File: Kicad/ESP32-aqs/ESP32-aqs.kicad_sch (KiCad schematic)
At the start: 28 parts, among them J2 JST connector SEN55, J3 ufl connector, J4 UART Connector, SW1 TC-1102-B-C-B, SW2 TC-1102-B-C-B, U1 LD1117S33TR_SOT223, U2 ESP32-WROOM-32, U3 SGP41-D-R4, U4 SX1276S8S+T-X1

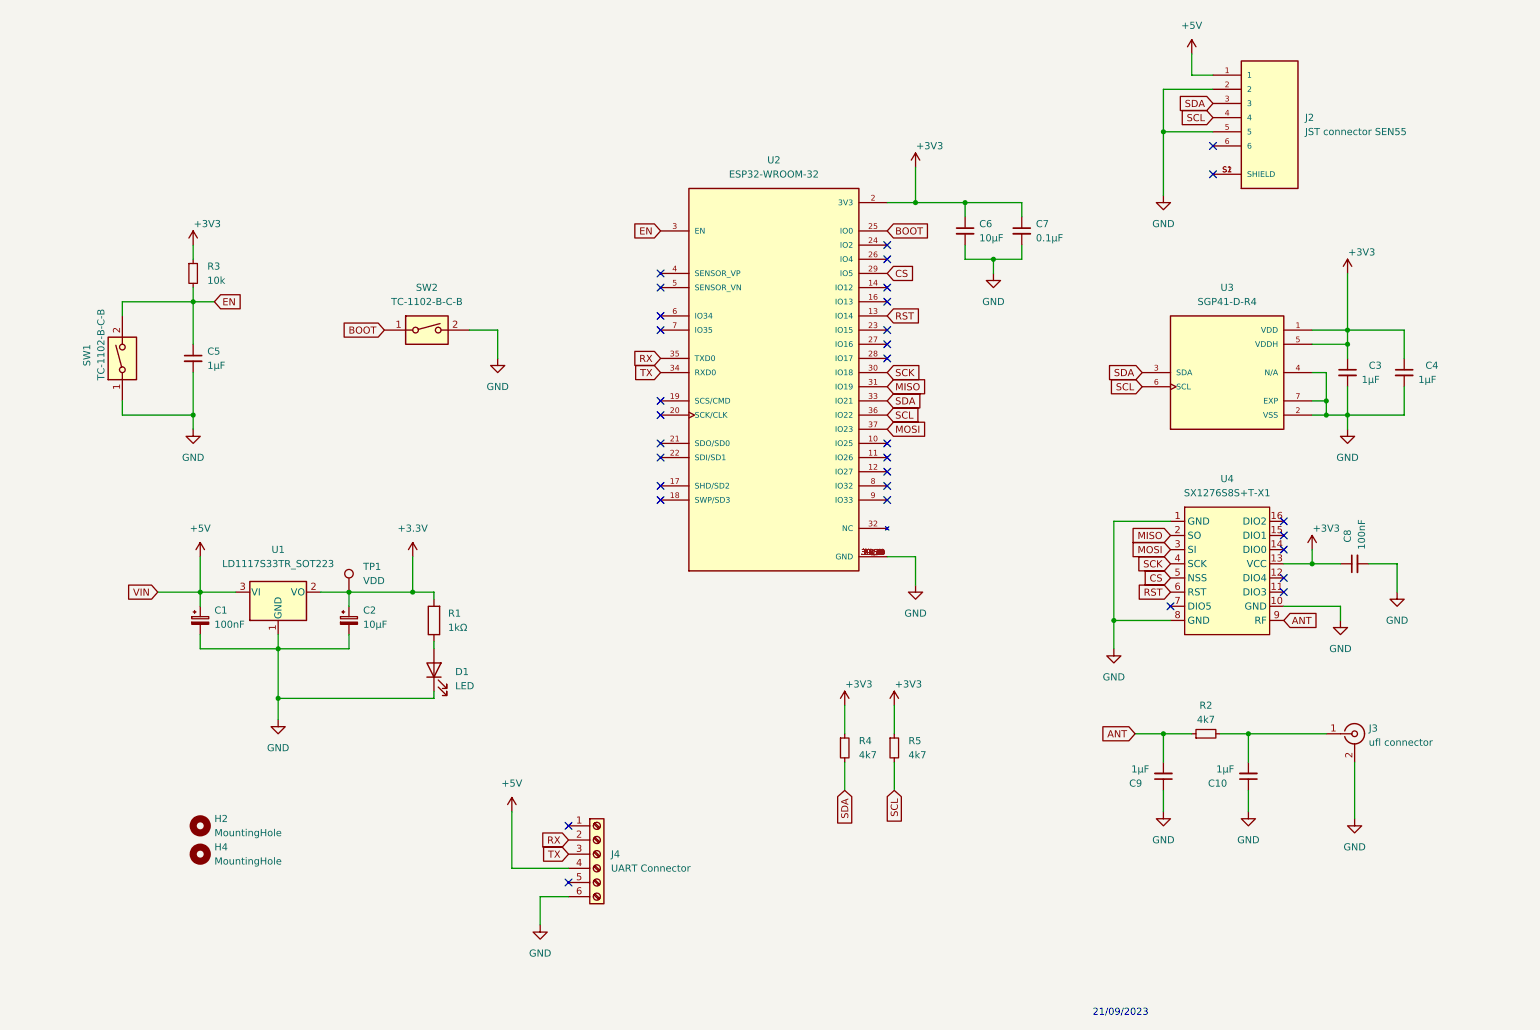
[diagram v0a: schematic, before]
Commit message: schematic v2
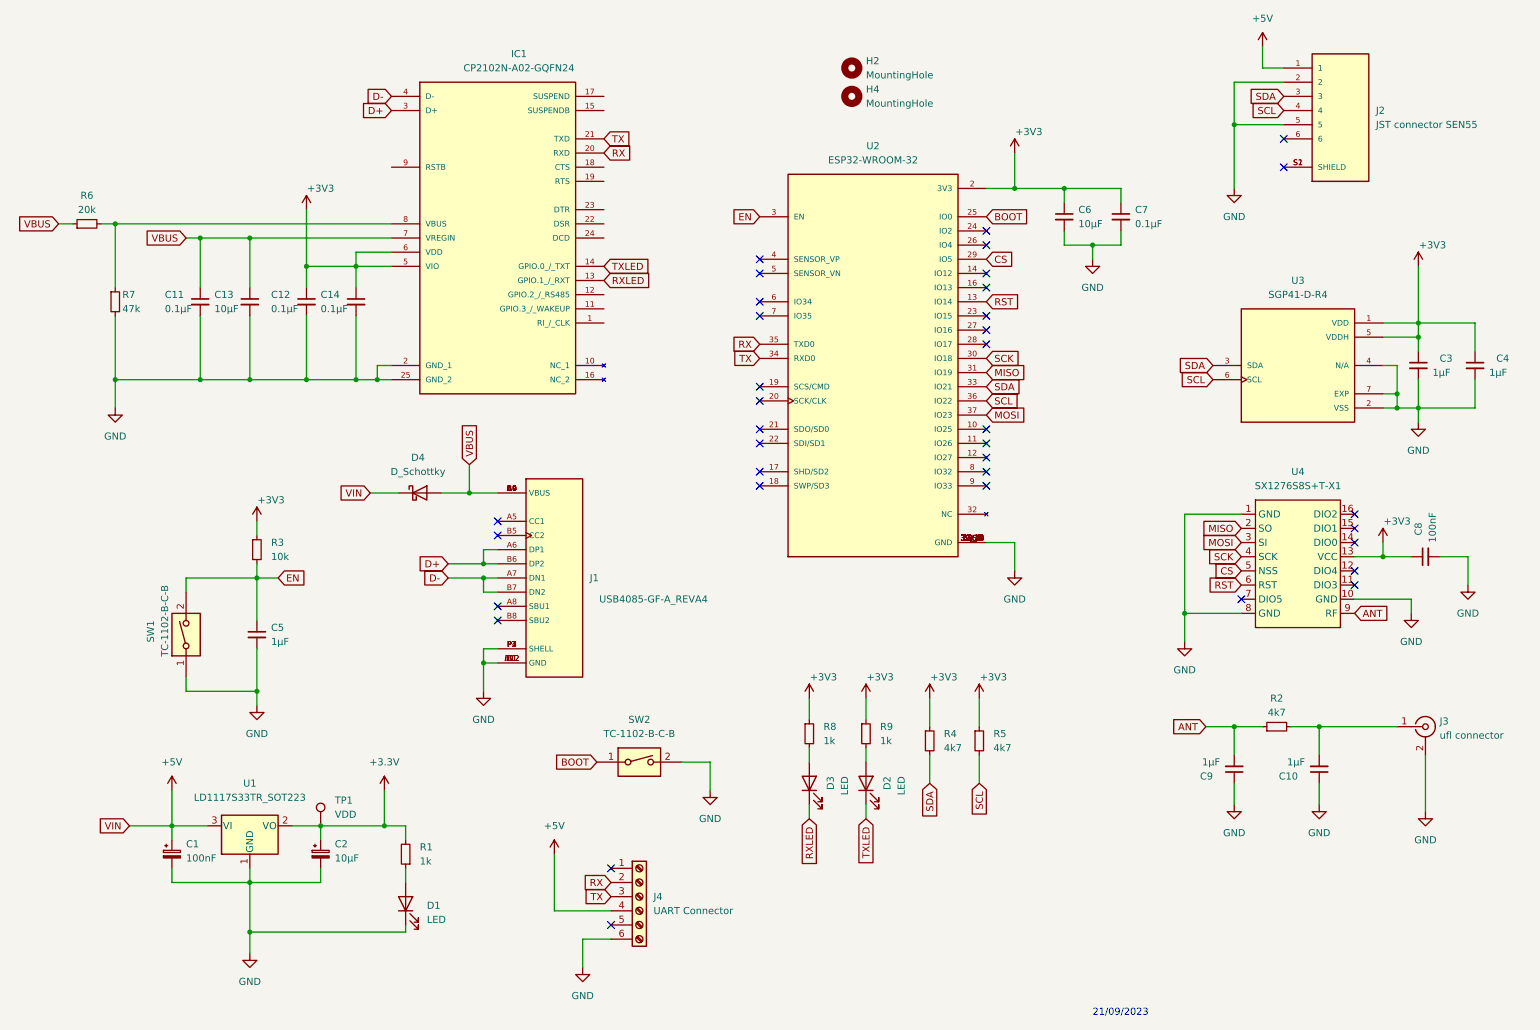
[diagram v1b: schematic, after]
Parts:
- removed R1: 1kΩ, Resistor_SMD:R_0805_2012Metric_Pad1.20x1.40mm_HandSolder, symbol Device:R
- added C11, C12, C14: 0.1µF, Capacitor_SMD:C_0805_2012Metric_Pad1.18x1.45mm_HandSolder, symbol Device:C_Small
- added C13: 10µF, Capacitor_SMD:C_0805_2012Metric_Pad1.18x1.45mm_HandSolder, symbol Device:C_Small
- added D2, D3: LED, LED_SMD:LED_0805_2012Metric_Pad1.15x1.40mm_HandSolder, symbol Device:LED
- added D4: D_Schottky, ESP32-aqs:SOD-123FL, symbol Device:D_Schottky
- added IC1: CP2102N-A02-GQFN24, ESP32-aqs:QFN50P400X400X80-25N, symbol ESP32-aqs:CP2102N-A02-GQFN24
- added J1: USB4085-GF-A_REVA4, ESP32-aqs:GCT_USB4085-GF-A_REVA4, symbol ESP32-aqs:USB-C_Connector
- added R1, R8, R9: 1k, Resistor_SMD:R_0805_2012Metric_Pad1.20x1.40mm_HandSolder, symbol Device:R_Small
- added R6: 20k, Resistor_SMD:R_0805_2012Metric_Pad1.20x1.40mm_HandSolder, symbol Device:R_Small
- added R7: 47k, Resistor_SMD:R_0805_2012Metric_Pad1.20x1.40mm_HandSolder, symbol Device:R_Small
- U3: footprint Library:SGP41 -> ESP32-aqs:XDCR_SGP41-D-R4
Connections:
- net +3V3: now also C12.1, C14.1, IC1.5 (VIO), IC1.6 (VDD), R1.2, R8.1, R9.1
- net +5V: now also D4.1 (K)
- net GND: now also C11.2, C12.2, C13.2, C14.2, IC1.2 (GND_1), IC1.25 (GND_2), J1.A1 (GND), J1.A12 (GND), J1.B1 (GND), J1.B12 (GND), J1.P1 (SHELL), J1.P2 (SHELL), J1.P3 (SHELL), J1.P4 (SHELL), R7.2
- net RX: now also IC1.20 (RXD)
- net TX: now also IC1.21 (TXD)
- net at D1.2 (A): now also R1.1
- new net: IC1.8 (VBUS), R6.2, R7.1
- new net: D2.2 (A), R9.2
- new net: D3.2 (A), R8.2
- new net D+: IC1.3 (D+), J1.A6 (DP1), J1.B6 (DP2)
- new net D-: IC1.4 (D-), J1.A7 (DN1), J1.B7 (DN2)
- new net RXLED: D3.1 (K), IC1.13 (GPIO.1_/_RXT)
- new net TXLED: D2.1 (K), IC1.14 (GPIO.0_/_TXT)
- new net VBUS: C11.1, C13.1, D4.2 (A), IC1.7 (VREGIN), J1.A4 (VBUS), J1.A9 (VBUS), J1.B4 (VBUS), J1.B9 (VBUS), R6.1
- no-connect marks 32 -> 36
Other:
- moved on the sheet: C1, C10, C2, C3, C4, C5, C6, C7, C8, C9, D1, H2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
